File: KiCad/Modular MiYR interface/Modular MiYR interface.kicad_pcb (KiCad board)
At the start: 4 copper layers, 65.5 x 107 mm, 86 parts, among them CN1 Conn_02x40_Odd_Even, CN2 Conn_02x40_Odd_Even, J1 FPC-05FB-50PH20, J2 FPC-05FB-50PH20, J3 FPC-05FB-50PH20, J4 FPC-05FB-50PH20, J5 FPC-05FB-50PH20, J6 24v, J7 Conn_01x08_Socket, M1 Fan, U1 TPS54202DDC, U2 TPS54202DDC, U3 TPS54202DDC

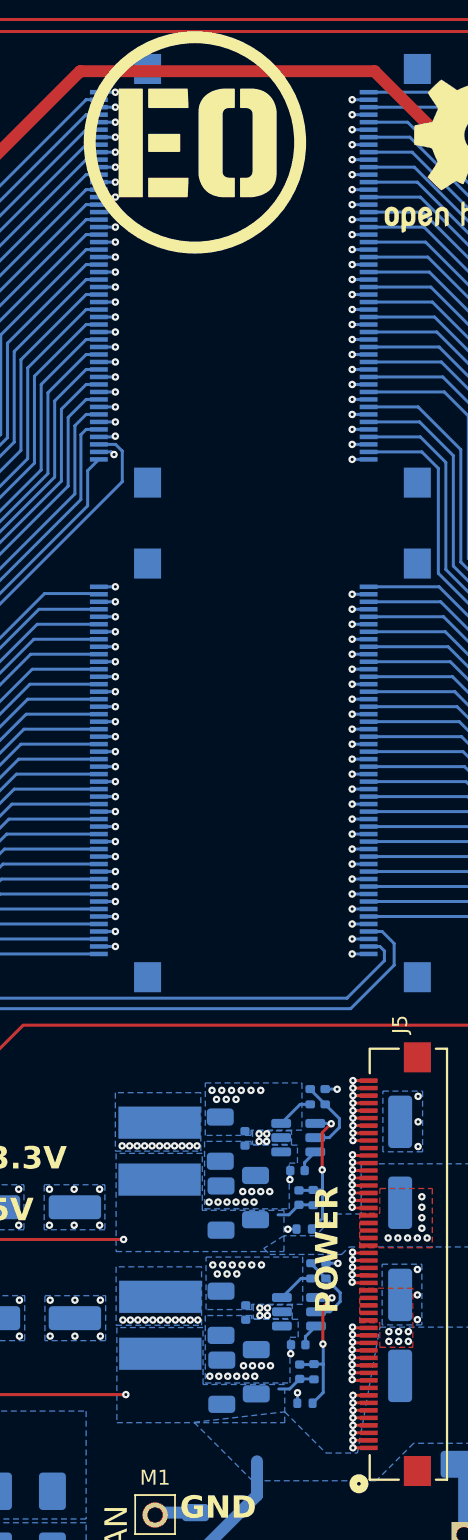
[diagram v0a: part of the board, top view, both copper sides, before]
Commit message: update
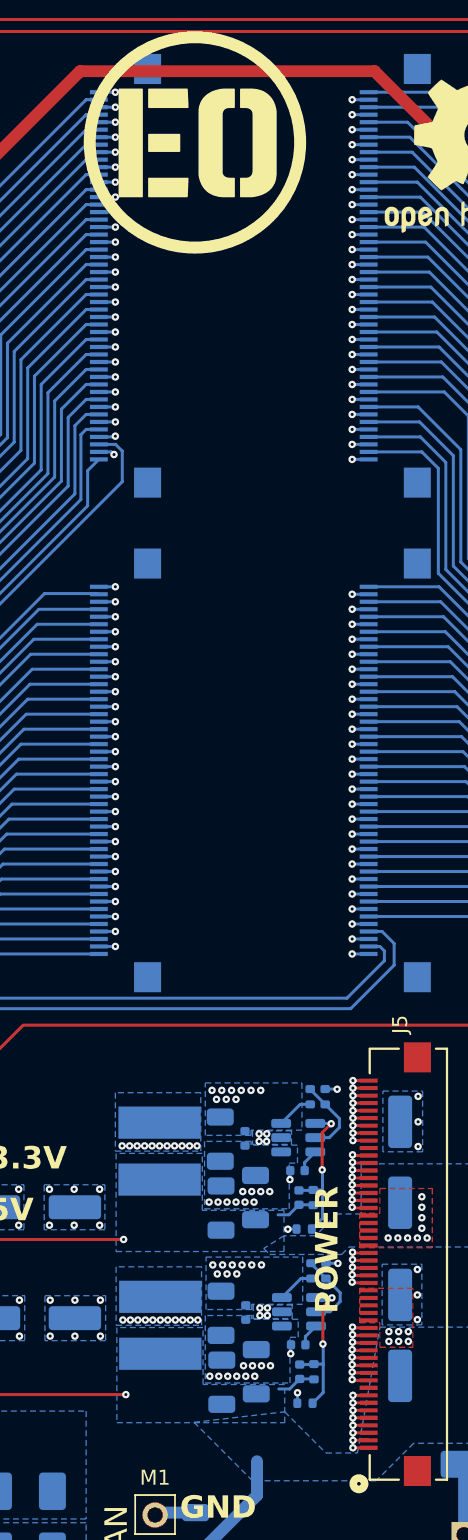
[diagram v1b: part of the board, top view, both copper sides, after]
